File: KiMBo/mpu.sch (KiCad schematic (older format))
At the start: 14 parts, among them U1 OSD3358

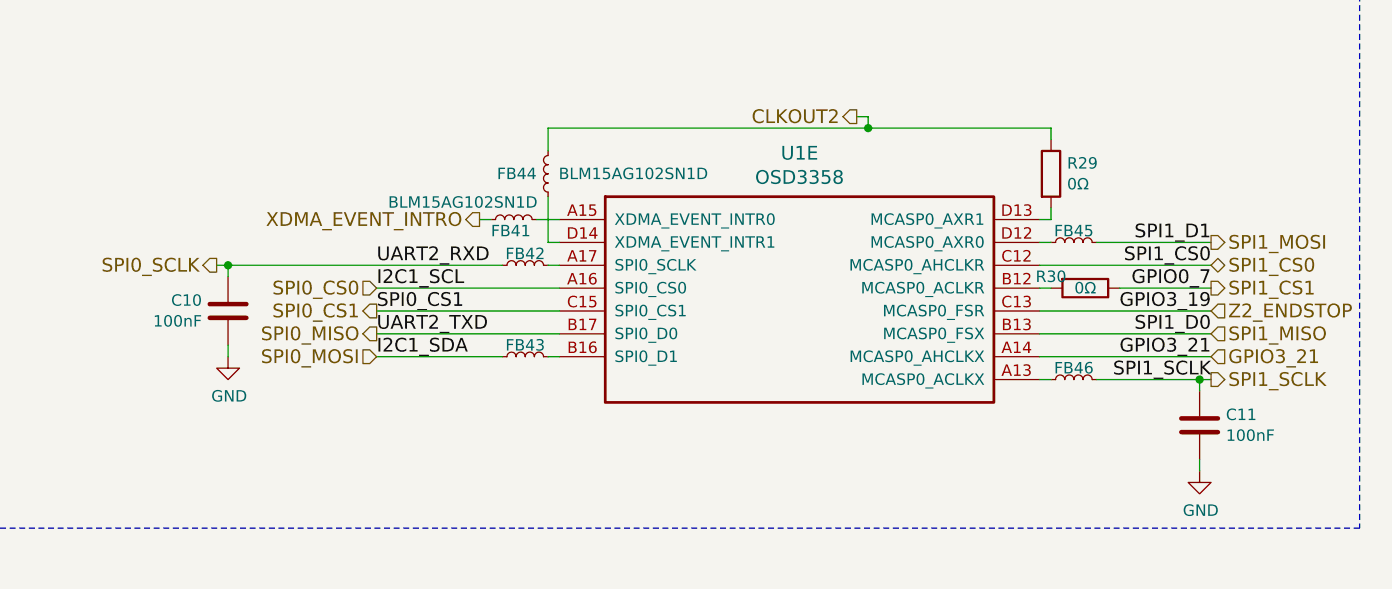
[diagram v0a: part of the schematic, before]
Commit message: Complete parallel data bus routing from the eMMC to the CPU
Center the SiP on the PCB

Add LPFs at the I2Cs' SCL outputs
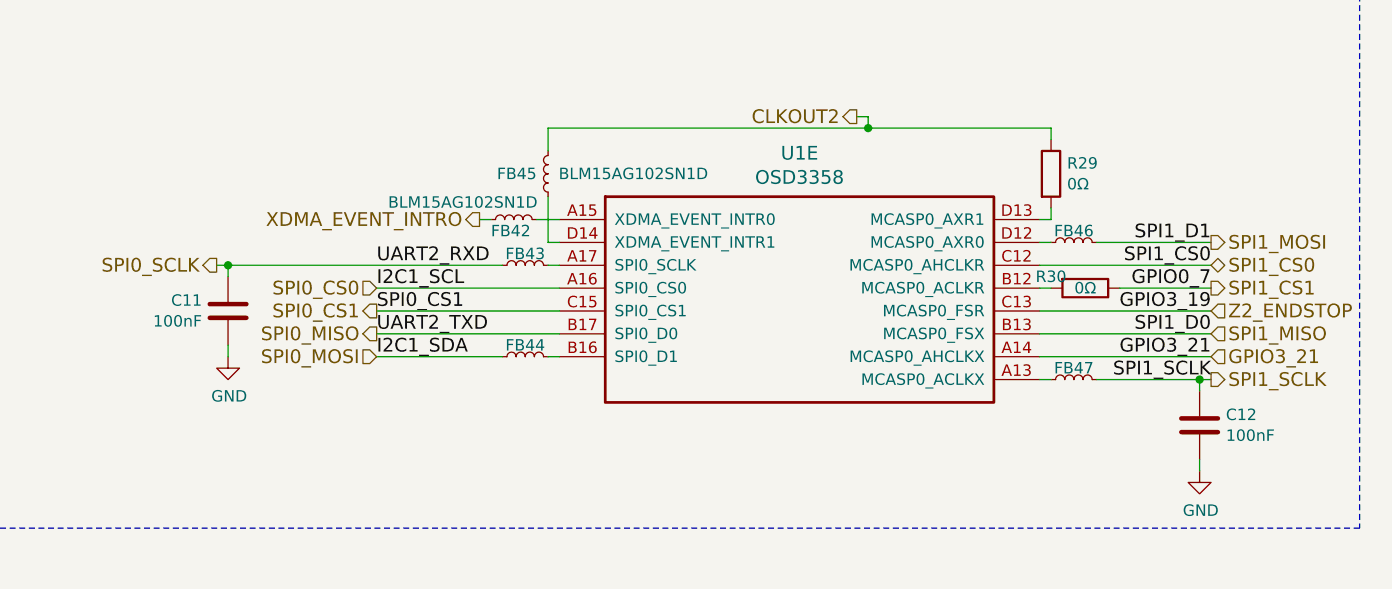
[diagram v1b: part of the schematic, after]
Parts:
- renumbered C10 to C11, C11 to C12, FB41 to FB42, FB42 to FB43, FB43 to FB44, FB44 to FB45, FB45 to FB46, FB46 to FB47
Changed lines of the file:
@@
 $EndComp
 $Comp
-L GND #PWR083
+L GND #PWR084
 U 1 1 584B7680
 P 6100 7850
-F 0 "#PWR083" H 6100 7600 50  0001 C CNN
+F 0 "#PWR084" H 6100 7600 50  0001 C CNN
 F 1 "GND" H 6105 7677 50  0000 C CNN
 F 2 "" H 6100 7850 50  0000 C CNN
@@
 SPI1_CS1
 $Comp
-L VDD_ADC #PWR084
+L VDD_ADC #PWR085
 U 1 1 59E85302
 P 7000 7650
-F 0 "#PWR084" H 7150 7600 50  0001 C CNN
+F 0 "#PWR085" H 7150 7600 50  0001 C CNN
 F 1 "VDD_ADC" H 7020 7793 50  0000 C CNN
 F 2 "" H 7000 7650 50  0000 C CNN
@@
 $EndComp
 $Comp
-L VDD_3V3B #PWR085
+L VDD_3V3B #PWR086
 U 1 1 59FC1115
 P 6100 7050
-F 0 "#PWR085" H 6100 6900 50  0001 C CNN
+F 0 "#PWR086" H 6100 6900 50  0001 C CNN
 F 1 "VDD_3V3B" H 6115 7223 50  0000 C CNN
 F 2 "" H 6100 7050 50  0000 C CNN
@@
 $EndComp
 $Comp
-L GNDA #PWR086
+L GNDA #PWR087
 U 1 1 59FCC96D
 P 7050 6500
-F 0 "#PWR086" H 7050 6250 50  0001 C CNN
+F 0 "#PWR087" H 7050 6250 50  0001 C CNN
 F 1 "GNDA" H 7055 6327 50  0000 C CNN
 F 2 "" H 7050 6500 50  0000 C CNN
@@
 Internal 150Ω FB\nfrom E8 to VSS\nunused on Replicape
 $Comp
-L PWR_FLAG #FLG087
+L PWR_FLAG #FLG088
 U 1 1 59FD3D41
 P 7150 6400
-F 0 "#FLG087" H 7150 6495 50  0001 C CNN
+F 0 "#FLG088" H 7150 6495 50  0001 C CNN
 F 1 "PWR_FLAG" H 7150 6624 50  0000 C CNN
 F 2 "" H 7150 6400 50  0000 C CNN
@@
 SPI0_SCLK
 $Comp
-L INDUCTOR_Small FB44
+L INDUCTOR_Small FB45
 U 1 1 58CEF5B5
 P 8950 3650
-F 0 "FB44" H 9000 3650 50  0000 L CNN
+F 0 "FB45" H 9000 3650 50  0000 L CNN
 F 1 "BLM15AG102SN1D" H 8250 3650 50  0000 L CNN
 F 2 "Resistors_SMD:R_0402" H 8950 3650 50  0001 C CNN
@@
 $EndComp
 $Comp
-L INDUCTOR_Small FB41
+L INDUCTOR_Small FB42
 U 1 1 58CF0E6E
 P 8800 3850
-F 0 "FB41" V 8750 3750 50  0000 L CNN
+F 0 "FB42" V 8750 3750 50  0000 L CNN
 F 1 "BLM15AG102SN1D" V 8875 3300 50  0000 L CNN
 F 2 "Resistors_SMD:R_0402" H 8800 3850 50  0001 C CNN
@@
 	8650 3850 8700 3850
 $Comp
-L INDUCTOR_Small FB46
+L INDUCTOR_Small FB47
 U 1 1 59121B69
 P 11250 4550
-F 0 "FB46" V 11300 4550 50  0000 C CNN
+F 0 "FB47" V 11300 4550 50  0000 C CNN
 F 1 "MMZ1608A252BTA00" V 11200 4550 50  0001 C CNN
 F 2 "KiMBo:Ferrite_Bead_0603" H 11250 4550 50  0001 C CNN
@@
 $EndComp
 $Comp
-L INDUCTOR_Small FB45
+L INDUCTOR_Small FB46
 U 1 1 59121BDD
 P 11250 3950
-F 0 "FB45" V 11300 3950 50  0000 C CNN
+F 0 "FB46" V 11300 3950 50  0000 C CNN
 F 1 "MMZ1608A252BTA00" V 11200 3950 50  0001 C CNN
 F 2 "KiMBo:Ferrite_Bead_0603" H 11250 3950 50  0001 C CNN
@@
 	11350 3950 11850 3950
 $Comp
-L INDUCTOR_Small FB42
+L INDUCTOR_Small FB43
 U 1 1 591407CC
 P 8850 4050
-F 0 "FB42" V 8900 4050 50  0000 C CNN
+F 0 "FB43" V 8900 4050 50  0000 C CNN
 F 1 "MMZ1608A252BTA00" V 8800 4050 50  0001 C CNN
 F 2 "KiMBo:Ferrite_Bead_0603" H 8850 4050 50  0001 C CNN
@@
 $EndComp
 $Comp
-L INDUCTOR_Small FB43
+L INDUCTOR_Small FB44
 U 1 1 59140942
 P 8850 4450
-F 0 "FB43" V 8900 4450 50  0000 C CNN
+F 0 "FB44" V 8900 4450 50  0000 C CNN
 F 1 "MMZ1608A252BTA00" V 8800 4450 50  0001 C CNN
 F 2 "KiMBo:Ferrite_Bead_0603" H 8850 4450 50  0001 C CNN
@@
 	8750 4450 8200 4450
 $Comp
-L C C10
+L C C11
 U 1 1 59301CCA
 P 7550 4250
-F 0 "C10" H 7664 4296 50  0000 L CNN
+F 0 "C11" H 7664 4296 50  0000 L CNN
 F 1 "100nF" H 7664 4205 50  0000 L CNN
 F 2 "Capacitors_SMD:C_0603" H 7664 4159 50  0001 L CNN
@@
 Connection ~ 7550 4050
 $Comp
-L GND #PWR088
+L GND #PWR089
 U 1 1 59301E33
 P 7550 4450
-F 0 "#PWR088" H 7550 4200 50  0001 C CNN
+F 0 "#PWR089" H 7550 4200 50  0001 C CNN
 F 1 "GND" H 7555 4277 50  0000 C CNN
 F 2 "" H 7550 4450 50  0000 C CNN
@@
 	7550 4450 7550 4400
 $Comp
-L C C11
+L C C12
 U 1 1 59302624
 P 11800 4750
-F 0 "C11" H 11915 4796 50  0000 L CNN
+F 0 "C12" H 11915 4796 50  0000 L CNN
 F 1 "100nF" H 11915 4705 50  0000 L CNN
 F 2 "Capacitors_SMD:C_0603" H 11915 4659 50  0001 L CNN
@@
 Connection ~ 11800 4550
 $Comp
-L GND #PWR089
+L GND #PWR090
 U 1 1 59302949
 P 11800 4950
-F 0 "#PWR089" H 11800 4700 50  0001 C CNN
+F 0 "#PWR090" H 11800 4700 50  0001 C CNN
 F 1 "GND" H 11805 4777 50  0000 C CNN
 F 2 "" H 11800 4950 50  0000 C CNN

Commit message: Routing open-drain output inverters, SOT-5 I2C EEPROM, begin adding bypass caps around the eMMC
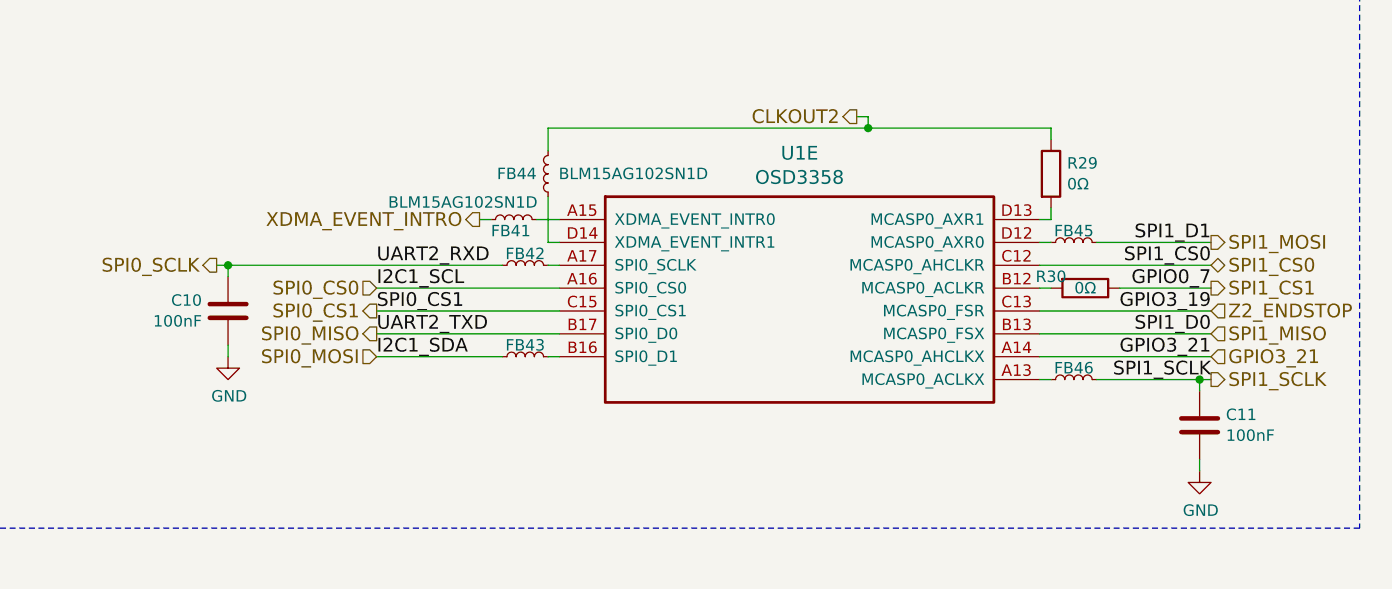
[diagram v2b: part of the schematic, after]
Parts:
- renumbered C11 to C10, C12 to C11, FB42 to FB41, FB43 to FB42, FB44 to FB43, FB45 to FB44, FB46 to FB45, FB47 to FB46
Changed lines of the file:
@@
 $EndComp
 $Comp
-L GND #PWR084
+L GND #PWR083
 U 1 1 584B7680
 P 6100 7850
-F 0 "#PWR084" H 6100 7600 50  0001 C CNN
+F 0 "#PWR083" H 6100 7600 50  0001 C CNN
 F 1 "GND" H 6105 7677 50  0000 C CNN
 F 2 "" H 6100 7850 50  0000 C CNN
@@
 SPI1_CS1
 $Comp
-L VDD_ADC #PWR085
+L VDD_ADC #PWR084
 U 1 1 59E85302
 P 7000 7650
-F 0 "#PWR085" H 7150 7600 50  0001 C CNN
+F 0 "#PWR084" H 7150 7600 50  0001 C CNN
 F 1 "VDD_ADC" H 7020 7793 50  0000 C CNN
 F 2 "" H 7000 7650 50  0000 C CNN
@@
 $EndComp
 $Comp
-L VDD_3V3B #PWR086
+L VDD_3V3B #PWR085
 U 1 1 59FC1115
 P 6100 7050
-F 0 "#PWR086" H 6100 6900 50  0001 C CNN
+F 0 "#PWR085" H 6100 6900 50  0001 C CNN
 F 1 "VDD_3V3B" H 6115 7223 50  0000 C CNN
 F 2 "" H 6100 7050 50  0000 C CNN
@@
 $EndComp
 $Comp
-L GNDA #PWR087
+L GNDA #PWR086
 U 1 1 59FCC96D
 P 7050 6500
-F 0 "#PWR087" H 7050 6250 50  0001 C CNN
+F 0 "#PWR086" H 7050 6250 50  0001 C CNN
 F 1 "GNDA" H 7055 6327 50  0000 C CNN
 F 2 "" H 7050 6500 50  0000 C CNN
@@
 Internal 150Ω FB\nfrom E8 to VSS\nunused on Replicape
 $Comp
-L PWR_FLAG #FLG088
+L PWR_FLAG #FLG087
 U 1 1 59FD3D41
 P 7150 6400
-F 0 "#FLG088" H 7150 6495 50  0001 C CNN
+F 0 "#FLG087" H 7150 6495 50  0001 C CNN
 F 1 "PWR_FLAG" H 7150 6624 50  0000 C CNN
 F 2 "" H 7150 6400 50  0000 C CNN
@@
 SPI0_SCLK
 $Comp
-L INDUCTOR_Small FB45
+L INDUCTOR_Small FB44
 U 1 1 58CEF5B5
 P 8950 3650
-F 0 "FB45" H 9000 3650 50  0000 L CNN
+F 0 "FB44" H 9000 3650 50  0000 L CNN
 F 1 "BLM15AG102SN1D" H 8250 3650 50  0000 L CNN
 F 2 "Resistors_SMD:R_0402" H 8950 3650 50  0001 C CNN
@@
 $EndComp
 $Comp
-L INDUCTOR_Small FB42
+L INDUCTOR_Small FB41
 U 1 1 58CF0E6E
 P 8800 3850
-F 0 "FB42" V 8750 3750 50  0000 L CNN
+F 0 "FB41" V 8750 3750 50  0000 L CNN
 F 1 "BLM15AG102SN1D" V 8875 3300 50  0000 L CNN
 F 2 "Resistors_SMD:R_0402" H 8800 3850 50  0001 C CNN
@@
 	8650 3850 8700 3850
 $Comp
-L INDUCTOR_Small FB47
+L INDUCTOR_Small FB46
 U 1 1 59121B69
 P 11250 4550
-F 0 "FB47" V 11300 4550 50  0000 C CNN
+F 0 "FB46" V 11300 4550 50  0000 C CNN
 F 1 "MMZ1608A252BTA00" V 11200 4550 50  0001 C CNN
 F 2 "KiMBo:Ferrite_Bead_0603" H 11250 4550 50  0001 C CNN
@@
 $EndComp
 $Comp
-L INDUCTOR_Small FB46
+L INDUCTOR_Small FB45
 U 1 1 59121BDD
 P 11250 3950
-F 0 "FB46" V 11300 3950 50  0000 C CNN
+F 0 "FB45" V 11300 3950 50  0000 C CNN
 F 1 "MMZ1608A252BTA00" V 11200 3950 50  0001 C CNN
 F 2 "KiMBo:Ferrite_Bead_0603" H 11250 3950 50  0001 C CNN
@@
 	11350 3950 11850 3950
 $Comp
-L INDUCTOR_Small FB43
+L INDUCTOR_Small FB42
 U 1 1 591407CC
 P 8850 4050
-F 0 "FB43" V 8900 4050 50  0000 C CNN
+F 0 "FB42" V 8900 4050 50  0000 C CNN
 F 1 "MMZ1608A252BTA00" V 8800 4050 50  0001 C CNN
 F 2 "KiMBo:Ferrite_Bead_0603" H 8850 4050 50  0001 C CNN
@@
 $EndComp
 $Comp
-L INDUCTOR_Small FB44
+L INDUCTOR_Small FB43
 U 1 1 59140942
 P 8850 4450
-F 0 "FB44" V 8900 4450 50  0000 C CNN
+F 0 "FB43" V 8900 4450 50  0000 C CNN
 F 1 "MMZ1608A252BTA00" V 8800 4450 50  0001 C CNN
 F 2 "KiMBo:Ferrite_Bead_0603" H 8850 4450 50  0001 C CNN
@@
 	8750 4450 8200 4450
 $Comp
-L C C11
+L C C10
 U 1 1 59301CCA
 P 7550 4250
-F 0 "C11" H 7664 4296 50  0000 L CNN
+F 0 "C10" H 7664 4296 50  0000 L CNN
 F 1 "100nF" H 7664 4205 50  0000 L CNN
 F 2 "Capacitors_SMD:C_0603" H 7664 4159 50  0001 L CNN
@@
 Connection ~ 7550 4050
 $Comp
-L GND #PWR089
+L GND #PWR088
 U 1 1 59301E33
 P 7550 4450
-F 0 "#PWR089" H 7550 4200 50  0001 C CNN
+F 0 "#PWR088" H 7550 4200 50  0001 C CNN
 F 1 "GND" H 7555 4277 50  0000 C CNN
 F 2 "" H 7550 4450 50  0000 C CNN
@@
 	7550 4450 7550 4400
 $Comp
-L C C12
+L C C11
 U 1 1 59302624
 P 11800 4750
-F 0 "C12" H 11915 4796 50  0000 L CNN
+F 0 "C11" H 11915 4796 50  0000 L CNN
 F 1 "100nF" H 11915 4705 50  0000 L CNN
 F 2 "Capacitors_SMD:C_0603" H 11915 4659 50  0001 L CNN
@@
 Connection ~ 11800 4550
 $Comp
-L GND #PWR090
+L GND #PWR089
 U 1 1 59302949
 P 11800 4950
-F 0 "#PWR090" H 11800 4700 50  0001 C CNN
+F 0 "#PWR089" H 11800 4700 50  0001 C CNN
 F 1 "GND" H 11805 4777 50  0000 C CNN
 F 2 "" H 11800 4950 50  0000 C CNN
